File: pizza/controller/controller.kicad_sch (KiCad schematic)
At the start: 4 parts, among them SW1 Button A, SW2 Button B, SW3 Button Opt, SW4 SKRHAAE010

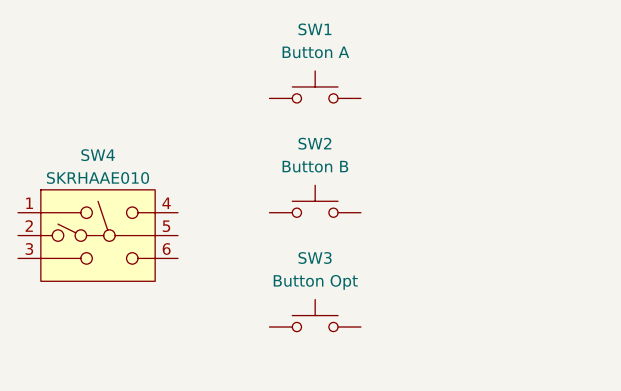
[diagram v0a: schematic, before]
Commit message: コントローラ基板が完成
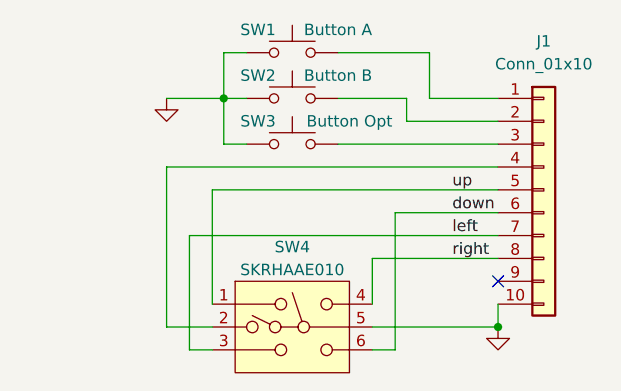
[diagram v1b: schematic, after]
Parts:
- added J1: Conn_01x10, Connector_PinHeader_2.54mm:PinHeader_1x10_P2.54mm_Horizontal, symbol Connector_Generic:Conn_01x10
- SW4: footprint (none) -> uchan:SKRHAAE010
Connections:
- net GND: now reaches SW2.1
- net GND: now also SW1.1, SW3.1, SW4.5, J1.10 (Pin_10)
- net at SW2.2: now also J1.2 (Pin_2)
- net at SW3.2: now also J1.3 (Pin_3)
- net at SW1.2: now also J1.1 (Pin_1)
- net up: now reaches SW4.1
- net up: now also J1.5 (Pin_5)
- net at SW4.2: now also J1.4 (Pin_4)
- net left: now reaches SW4.3
- net left: now also J1.7 (Pin_7)
- net right: now reaches SW4.4
- net right: now also J1.8 (Pin_8)
- net down: now reaches SW4.6
- net down: now also J1.6 (Pin_6)
- no-connect marks 0 -> 1
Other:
- moved on the sheet: SW1, SW2, SW3, SW4
